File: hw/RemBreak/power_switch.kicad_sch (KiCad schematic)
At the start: 27 parts, among them Q5 BC337, Q6 SiS415DNT, Q7 BC847, Q8 BC337, Q9 BC847, U10 MAX40200AUK, U5 BD4830FVE-TR, U6 L7805, U7 L7805, U8 XC6220B331MR, U9 MAX40200AUK

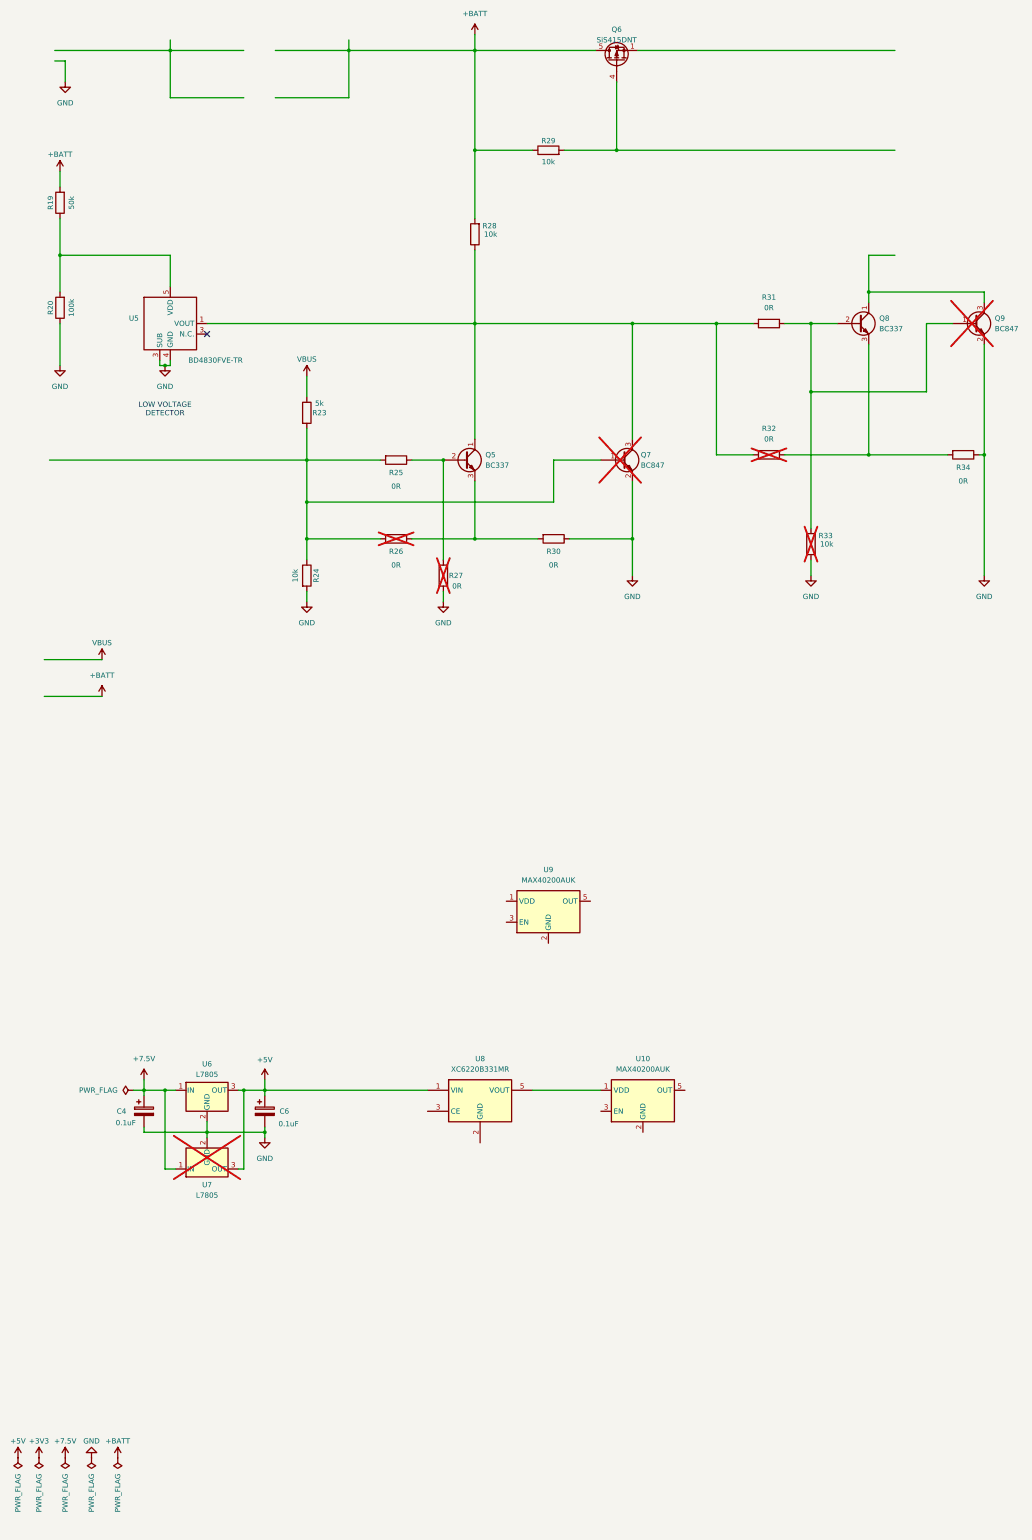
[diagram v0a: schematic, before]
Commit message: schematics drawing in progress
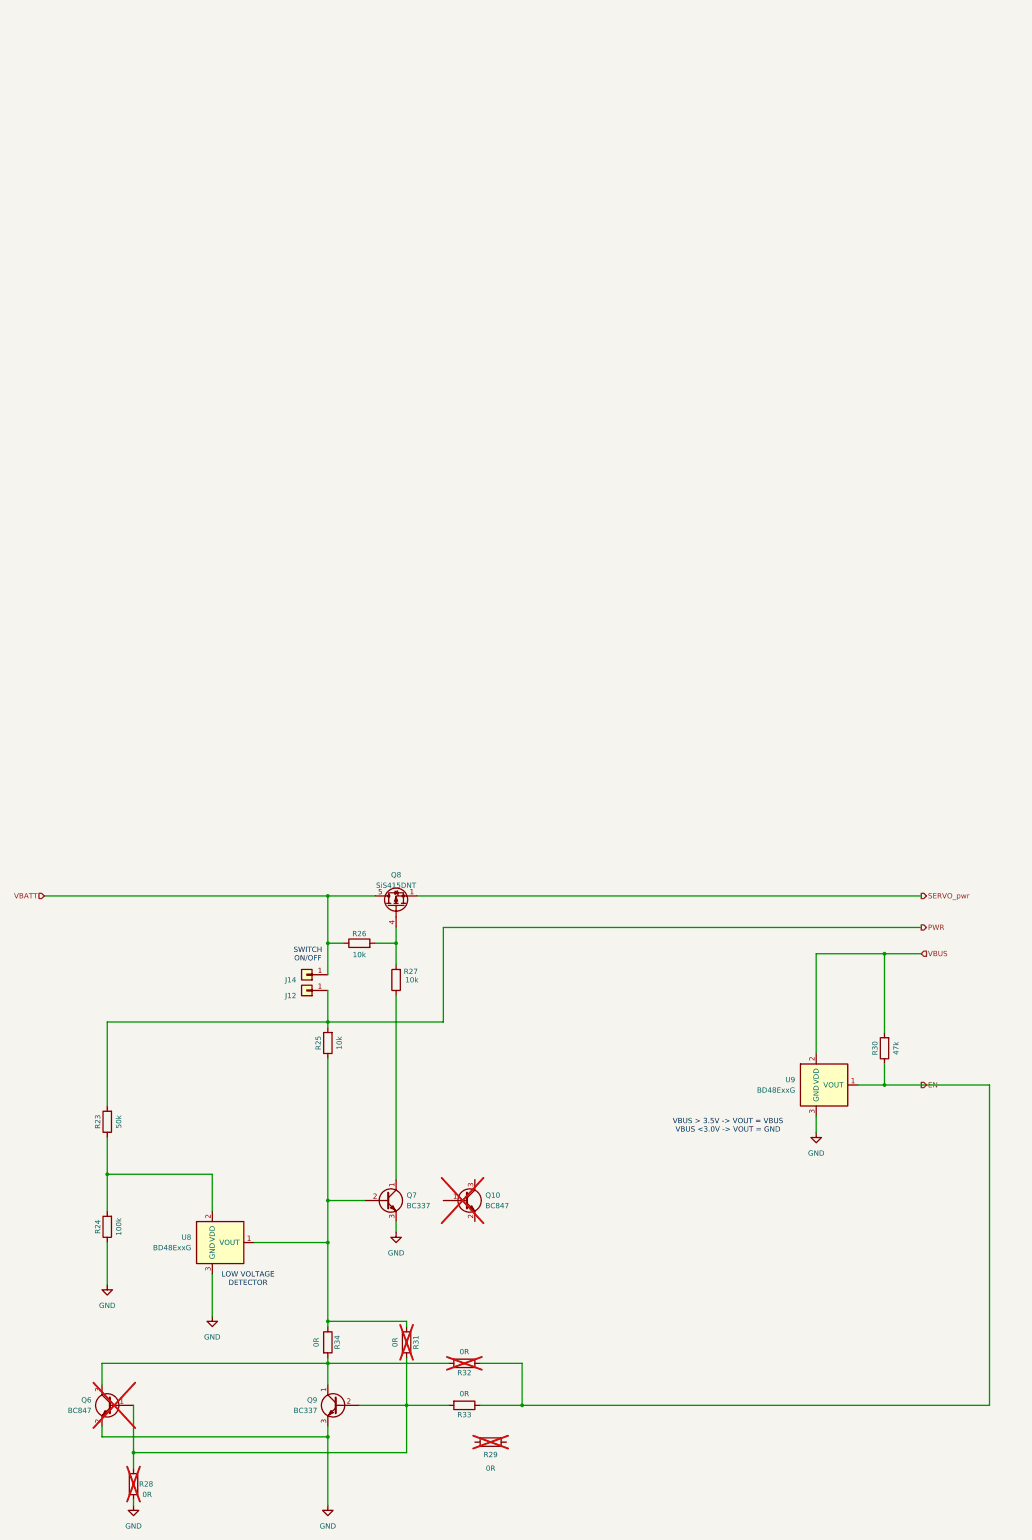
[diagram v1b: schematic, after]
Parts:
- removed C4, C6: 0.1uF, Capacitor_SMD:C_0805_2012Metric, symbol Device:C_Polarized
- removed Q7: BC847, Package_TO_SOT_SMD:SOT-23, symbol Transistor_BJT:BC847
- removed Q8: BC337, Package_TO_SOT_THT:TO-92_Inline, symbol Transistor_BJT:BC337
- removed R23: 5k, Resistor_SMD:R_0805_2012Metric, symbol Device:R
- removed R24, R28, R29: 10k, Resistor_SMD:R_0805_2012Metric, symbol Device:R
- removed U10, U9: MAX40200AUK, Package_TO_SOT_SMD:SOT-23-5, symbol Analog_Switch:MAX40200AUK
- removed U5: BD4830FVE-TR, Package_TO_SOT_SMD:VSOF5, symbol dodo-power:BD4830FVE-TR
- removed U6: L7805, Package_TO_SOT_SMD:TO-263-2, symbol Regulator_Linear:L7805
- removed U7: L7805, Package_TO_SOT_THT:TO-220-3_Horizontal_TabDown, symbol Regulator_Linear:L7805
- removed U8: XC6220B331MR, Package_TO_SOT_SMD:SOT-23-5, symbol Regulator_Linear:XC6220B331MR
- added J12, J14: Conn_01x01, TestPoint:TestPoint_Pad_2.5x2.5mm, symbol Connector_Generic:Conn_01x01
- added Q6: BC847, Package_TO_SOT_SMD:SOT-23, symbol Transistor_BJT:BC847
- added Q9: BC337, Package_TO_SOT_THT:TO-92_Inline, symbol Transistor_BJT:BC337
- added R26, R27: 10k, Resistor_SMD:R_0805_2012Metric, symbol Device:R
- added U8, U9: BD48ExxG, Package_TO_SOT_SMD:SOT-23-5, symbol Power_Management:BD48ExxG
- R25: value 0R -> 10k
- R30: value 0R -> 47k
- R31: now not fitted
- R33: value 10k -> 0R; now fitted
- renumbered Q9 to Q10, Q5 to Q7, Q6 to Q8, R19 to R23, R20 to R24, R27 to R28, R26 to R29
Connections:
- net GND: now also Q7.3 (E), Q6.2 (E), Q9.3 (E), U8.3 (GND), U9.3 (GND); no longer Q10.2 (E), R30.1, R33.1, R34.1
- net VBUS: now also R30.2, U9.2 (VDD)
- net at R29.2: no longer R25.2
- net at R23.1, R24.2: now also U8.2 (VDD)
- net at R34.2: now also R32.2, Q6.3 (C), Q9.1 (C); no longer R32.1
- net at Q7.2 (B), R25.1: now also R31.1, R34.1, U8.1 (VOUT); no longer R28.1
- net SERVO_pwr: now reaches Q8.1 (S), Q8.2 (S), Q8.3 (S)
- net at Q8.4 (G): now also R26.2, R27.2
- net +BATT renamed PWR
- net PWR: now also R25.2, J12.1 (Pin_1); no longer Q8.5 (D)
- new net: Q6.1 (B), Q9.2 (B), R28.1, R31.2, R33.2
- new net: Q7.1 (C), R27.1
- new net EN: R30.1, R32.1, R33.1, U9.1 (VOUT)
- new net VBATT: J14.1 (Pin_1), Q8.5 (D), R26.1
- now unconnected: Q10.1 (B), R29.1
- no-connect marks 1 -> 0
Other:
- note added: "SWITCH ON/OFF"
- note added: "VBUS > 3.5V -> VOUT = VBUS VBUS <3.0V -> VOUT = GND"
- moved on the sheet: Q10, Q7, Q8, R23, R24, R28, R29
